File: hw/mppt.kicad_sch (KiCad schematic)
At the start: 11 parts

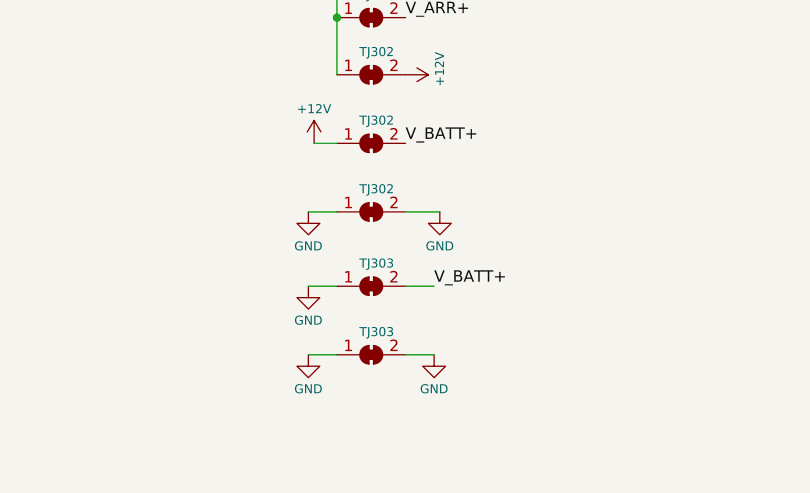
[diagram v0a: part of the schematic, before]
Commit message: hw changes
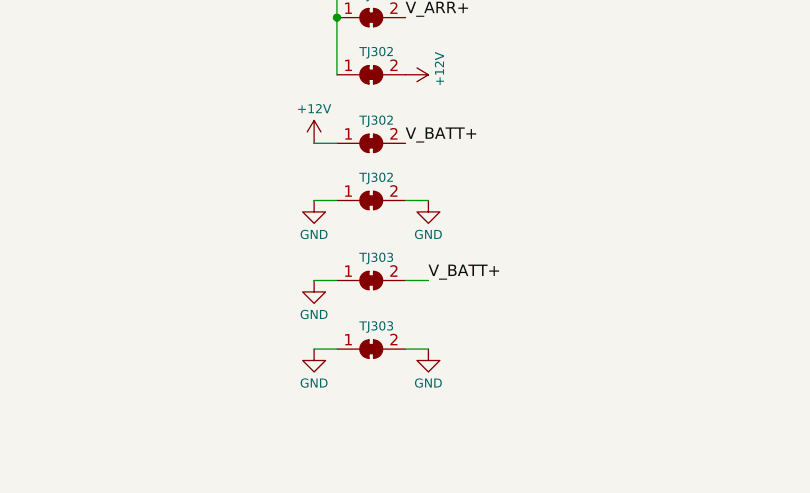
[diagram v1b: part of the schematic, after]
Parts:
- TJ302, TJ303: footprint mppt:1225_SMD -> footprints:1225_SMD
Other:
- moved on the sheet: TJ302, TJ303
